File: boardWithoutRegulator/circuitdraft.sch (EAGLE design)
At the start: 36 parts, among them IC1 BQ25887RGER, Q1 16 MHz

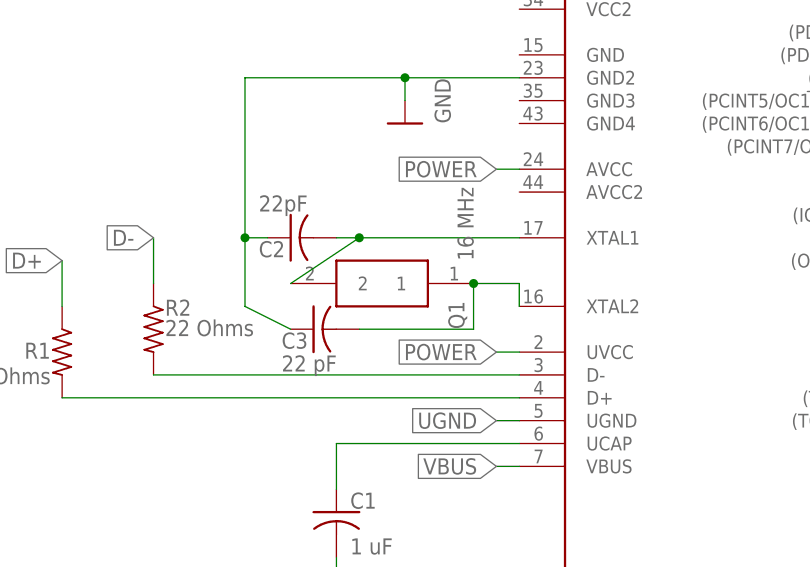
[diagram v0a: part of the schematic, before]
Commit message: Fixed it boii
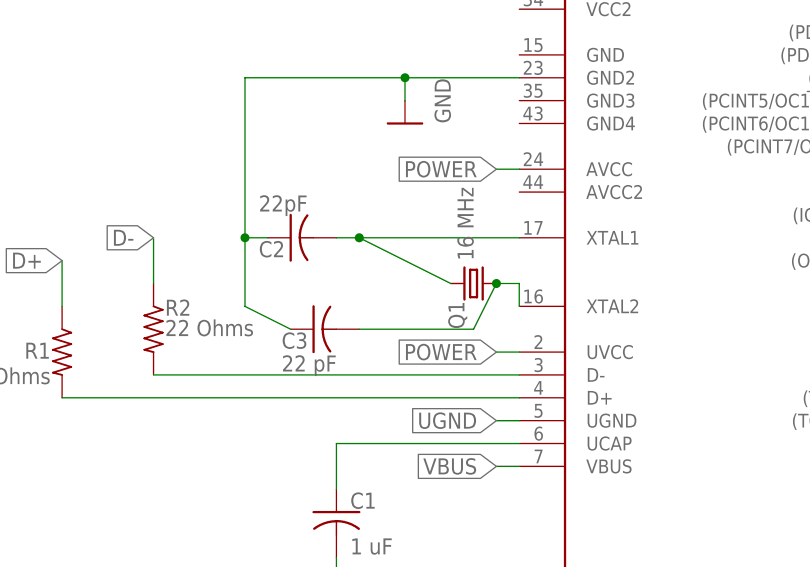
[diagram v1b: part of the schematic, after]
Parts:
- Q1: device SamacSys_Parts:ECS-160-18-23G-JGN-TR -> crystal-geyer_V1_0:KX-5
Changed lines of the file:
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@@
 <part name="AGND2" library="supply1" library_urn="urn:adsk.eagle:library:371" deviceset="GND" device=""/>
 <part name="AGND3" library="supply1" library_urn="urn:adsk.eagle:library:371" deviceset="GND" device=""/>
-<part name="Q1" library="SamacSys_Parts" deviceset="ECS-160-18-23G-JGN-TR" device="" value="16 MHz"/>
+<part name="Q1" library="crystal-geyer_V1_0" library_urn="urn:adsk.eagle:library:203" deviceset="KX" device="-5" package3d_urn="urn:adsk.eagle:package:11926/1" value="16 MHz"/>
 <part name="C2" library="rcl" library_urn="urn:adsk.eagle:library:334" deviceset="C-US" device="C0603" package3d_urn="urn:adsk.eagle:package:23616/2" value="22pF"/>
 <part name="C3" library="rcl" library_urn="urn:adsk.eagle:library:334" deviceset="C-US" device="C0603" package3d_urn="urn:adsk.eagle:package:23616/2" value="22 pF"/>
@@
 <wire x1="137.16" y1="149.86" x2="119.38" y2="149.86" width="0.1524" layer="91"/>
 <pinref part="Q1" gate="G$1" pin="2"/>
-<wire x1="119.38" y1="149.86" x2="111.76" y2="144.78" width="0.1524" layer="91"/>
+<wire x1="119.38" y1="149.86" x2="129.54" y2="144.78" width="0.1524" layer="91"/>
 <pinref part="C2" gate="G$1" pin="2"/>
 <wire x1="119.38" y1="149.86" x2="116.84" y2="149.86" width="0.1524" layer="91"/>
@@
 <pinref part="Q1" gate="G$1" pin="1"/>
 <wire x1="137.16" y1="142.24" x2="137.16" y2="144.78" width="0.1524" layer="91"/>
-<wire x1="137.16" y1="144.78" x2="132.08" y2="144.78" width="0.1524" layer="91"/>
-<wire x1="132.08" y1="144.78" x2="132.08" y2="139.7" width="0.1524" layer="91"/>
-<junction x="132.08" y="144.78"/>
+<wire x1="137.16" y1="144.78" x2="134.62" y2="144.78" width="0.1524" layer="91"/>
+<wire x1="134.62" y1="144.78" x2="132.08" y2="139.7" width="0.1524" layer="91"/>
+<junction x="134.62" y="144.78"/>
 <pinref part="C3" gate="G$1" pin="2"/>
 <wire x1="132.08" y1="139.7" x2="119.38" y2="139.7" width="0.1524" layer="91"/>
